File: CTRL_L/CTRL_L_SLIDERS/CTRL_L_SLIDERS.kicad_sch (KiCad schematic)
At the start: 1 part, among them J1 Conn_01x04_Socket

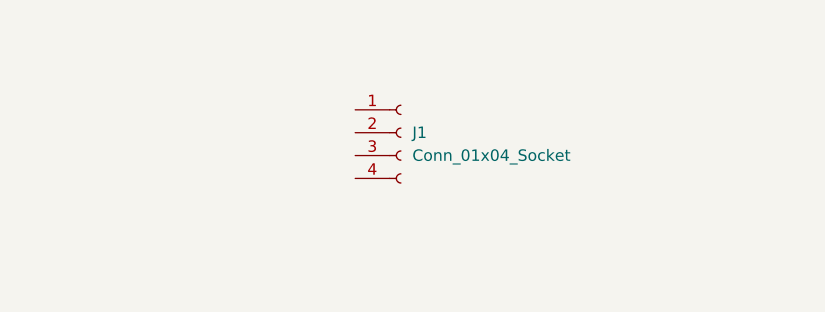
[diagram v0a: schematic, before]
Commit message: Finished Volume/Brightness Slider Daugherboard!
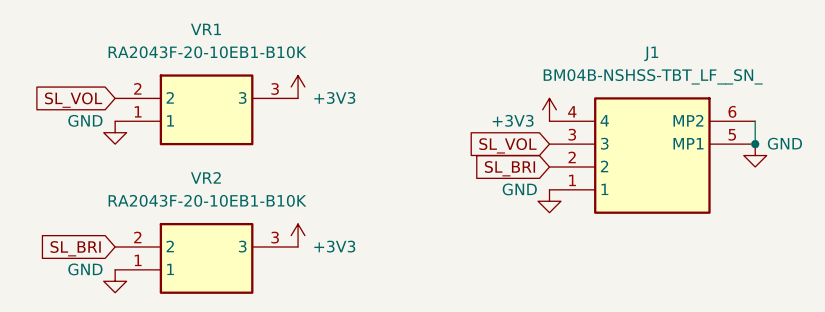
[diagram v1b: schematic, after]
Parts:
- removed J1: Conn_01x04_Socket, symbol Connector:Conn_01x04_Socket
- added J1: BM04B-NSHSS-TBT_LF__SN_, BM04BNSHSSTBTLFSN, symbol BM04B-NSHSS-TBT_LF__SN_:BM04B-NSHSS-TBT_LF__SN_
- added VR1, VR2: RA2043F-20-10EB1-B10K, RA2043F2010EB1B10K, symbol RA2043F-20-10EB1-B10K:RA2043F-20-10EB1-B10K
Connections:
- new net +3V3: J1.4, VR1.3, VR2.3
- new net GND: J1.1, J1.5 (MP1), J1.6 (MP2), VR1.1, VR2.1
- new net SL_BRI: J1.2, VR2.2
- new net SL_VOL: J1.3, VR1.2
